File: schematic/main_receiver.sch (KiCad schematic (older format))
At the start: 52 parts, among them J7 CONN_01X05, J8 raspberry_pi_3_header, Q2 NXP 2N7002, Q3 NXP 2N7002, Q4 NXP 2N7002, Q5 NXP 2N7002, U7 SX1301, Y1 ASEMB-133.3MHZ

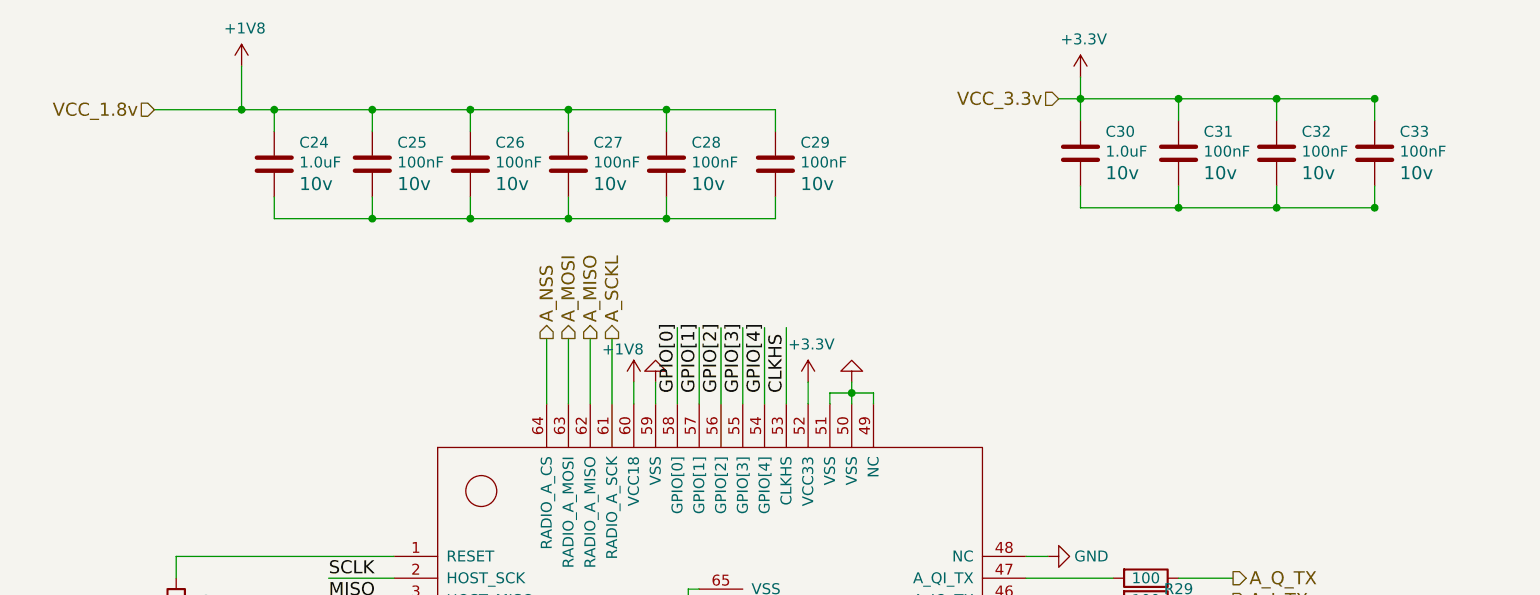
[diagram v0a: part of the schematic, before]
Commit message: Updates to schematic, components
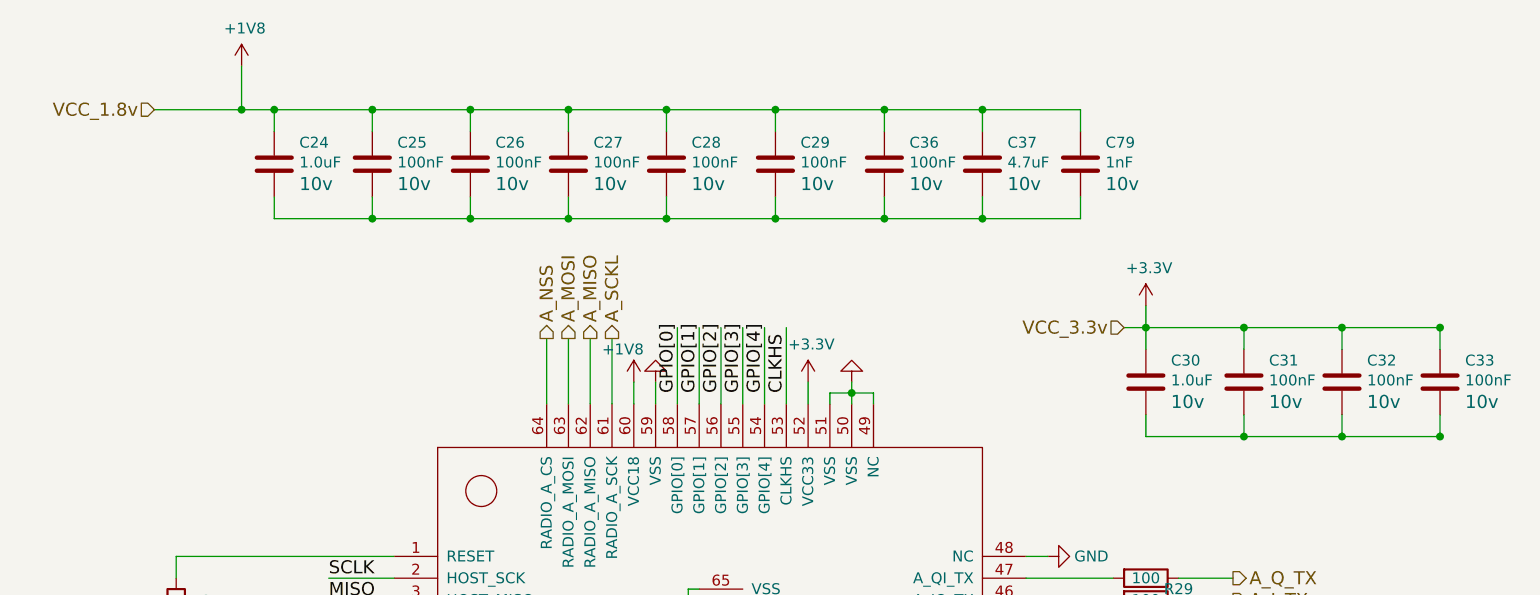
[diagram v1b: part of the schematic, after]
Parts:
- added C36: 100nF, symbol C
- added C37: 4.7uF, symbol C
- added C79: 1nF, symbol C
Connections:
- wire segments 191 -> 197
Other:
- moved on the sheet: C30, C31, C32, C33
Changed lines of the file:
@@
 L +3.3V #PWR055
 U 1 1 59B58145
-P 9000 900
-F 0 "#PWR055" H 9000 750 50  0001 C CNN
-F 1 "+3.3V" H 9015 1073 50  0000 C CNN
-F 2 "" H 9000 900 50  0001 C CNN
-F 3 "" H 9000 900 50  0001 C CNN
-	1    9000 900
-	1    0    0    -1
-$EndComp
-Text HLabel 8900 1000 0    60   Input ~ 0
+P 9300 1950
+F 0 "#PWR055" H 9300 1800 50  0001 C CNN
+F 1 "+3.3V" H 9315 2123 50  0000 C CNN
+F 2 "" H 9300 1950 50  0001 C CNN
+F 3 "" H 9300 1950 50  0001 C CNN
+	1    9300 1950
+	1    0    0    -1
+$EndComp
+Text HLabel 9200 2050 0    60   Input ~ 0
 VCC_3.3v
 Text HLabel 4750 1050 0    60   Input ~ 0
@@
 F 0 "C24" H 5415 1399 50  0000 L CNN
 F 1 "1.0uF" H 5415 1308 50  0000 L CNN
-F 2 "" H 5338 1150 50  0000 C CNN
+F 2 "" H 5338 1150 50  0001 C CNN
 F 3 "" H 5300 1300 50  0001 C CNN
 F 4 "10v" H 5415 1209 60  0000 L CNN "Voltage"
@@
 F 0 "C25" H 5865 1399 50  0000 L CNN
 F 1 "100nF" H 5865 1308 50  0000 L CNN
-F 2 "" H 5788 1150 50  0000 C CNN
+F 2 "" H 5788 1150 50  0001 C CNN
 F 3 "" H 5750 1300 50  0001 C CNN
 F 4 "10v" H 5865 1209 60  0000 L CNN "Voltage"
@@
 F 0 "C26" H 6315 1399 50  0000 L CNN
 F 1 "100nF" H 6315 1308 50  0000 L CNN
-F 2 "" H 6238 1150 50  0000 C CNN
+F 2 "" H 6238 1150 50  0001 C CNN
 F 3 "" H 6200 1300 50  0001 C CNN
 F 4 "10v" H 6315 1209 60  0000 L CNN "Voltage"
@@
 F 0 "C27" H 6765 1399 50  0000 L CNN
 F 1 "100nF" H 6765 1308 50  0000 L CNN
-F 2 "" H 6688 1150 50  0000 C CNN
+F 2 "" H 6688 1150 50  0001 C CNN
 F 3 "" H 6650 1300 50  0001 C CNN
 F 4 "10v" H 6765 1209 60  0000 L CNN "Voltage"
@@
 F 0 "C28" H 7215 1399 50  0000 L CNN
 F 1 "100nF" H 7215 1308 50  0000 L CNN
-F 2 "" H 7138 1150 50  0000 C CNN
+F 2 "" H 7138 1150 50  0001 C CNN
 F 3 "" H 7100 1300 50  0001 C CNN
 F 4 "10v" H 7215 1209 60  0000 L CNN "Voltage"
@@
 F 0 "C29" H 7715 1399 50  0000 L CNN
 F 1 "100nF" H 7715 1308 50  0000 L CNN
-F 2 "" H 7638 1150 50  0000 C CNN
+F 2 "" H 7638 1150 50  0001 C CNN
 F 3 "" H 7600 1300 50  0001 C CNN
 F 4 "10v" H 7715 1209 60  0000 L CNN "Voltage"
@@
 L C C30
 U 1 1 59B5D0C0
-P 9000 1250
-F 0 "C30" H 9115 1349 50  0000 L CNN
-F 1 "1.0uF" H 9115 1258 50  0000 L CNN
-F 2 "" H 9038 1100 50  0000 C CNN
-F 3 "" H 9000 1250 50  0001 C CNN
-F 4 "10v" H 9115 1159 60  0000 L CNN "Voltage"
-	1    9000 1250
+P 9300 2300
+F 0 "C30" H 9415 2399 50  0000 L CNN
+F 1 "1.0uF" H 9415 2308 50  0000 L CNN
+F 2 "" H 9338 2150 50  0001 C CNN
+F 3 "" H 9300 2300 50  0001 C CNN
+F 4 "10v" H 9415 2209 60  0000 L CNN "Voltage"
+	1    9300 2300
 	1    0    0    -1
 $EndComp
@@
 L C C31
 U 1 1 59B5D0C7
-P 9450 1250
-F 0 "C31" H 9565 1349 50  0000 L CNN
-F 1 "100nF" H 9565 1258 50  0000 L CNN
-F 2 "" H 9488 1100 50  0000 C CNN
-F 3 "" H 9450 1250 50  0001 C CNN
-F 4 "10v" H 9565 1159 60  0000 L CNN "Voltage"
-	1    9450 1250
+P 9750 2300
+F 0 "C31" H 9865 2399 50  0000 L CNN
+F 1 "100nF" H 9865 2308 50  0000 L CNN
+F 2 "" H 9788 2150 50  0001 C CNN
+F 3 "" H 9750 2300 50  0001 C CNN
+F 4 "10v" H 9865 2209 60  0000 L CNN "Voltage"
+	1    9750 2300
 	1    0    0    -1
 $EndComp
@@
 L C C32
 U 1 1 59B5D0CE
-P 9900 1250
-F 0 "C32" H 10015 1349 50  0000 L CNN
-F 1 "100nF" H 10015 1258 50  0000 L CNN
-F 2 "" H 9938 1100 50  0000 C CNN
-F 3 "" H 9900 1250 50  0001 C CNN
-F 4 "10v" H 10015 1159 60  0000 L CNN "Voltage"
-	1    9900 1250
+P 10200 2300
+F 0 "C32" H 10315 2399 50  0000 L CNN
+F 1 "100nF" H 10315 2308 50  0000 L CNN
+F 2 "" H 10238 2150 50  0001 C CNN
+F 3 "" H 10200 2300 50  0001 C CNN
+F 4 "10v" H 10315 2209 60  0000 L CNN "Voltage"
+	1    10200 2300
 	1    0    0    -1
 $EndComp
@@
 L C C33
 U 1 1 59B5D0D5
-P 10350 1250
-F 0 "C33" H 10465 1349 50  0000 L CNN
-F 1 "100nF" H 10465 1258 50  0000 L CNN
-F 2 "" H 10388 1100 50  0000 C CNN
-F 3 "" H 10350 1250 50  0001 C CNN
-F 4 "10v" H 10465 1159 60  0000 L CNN "Voltage"
-	1    10350 1250
+P 10650 2300
+F 0 "C33" H 10765 2399 50  0000 L CNN
+F 1 "100nF" H 10765 2308 50  0000 L CNN
+F 2 "" H 10688 2150 50  0001 C CNN
+F 3 "" H 10650 2300 50  0001 C CNN
+F 4 "10v" H 10765 2209 60  0000 L CNN "Voltage"
+	1    10650 2300
 	1    0    0    -1
 $EndComp
@@
 Connection ~ 3050 1150
 Wire Wire Line
-	4750 1050 7600 1050
+	4750 1050 9000 1050
 Wire Wire Line
 	5150 1050 5150 850
 Wire Wire Line
-	8900 1000 10350 1000
+	9200 2050 10650 2050
 Wire Wire Line
 	9300 4650 9200 4650
@@
 	7600 1550 7600 1450
 Wire Wire Line
-	5300 1550 7600 1550
+	5300 1550 9000 1550
 Wire Wire Line
 	5300 1550 5300 1450
@@
 Connection ~ 7100 1550
 Wire Wire Line
-	9450 1000 9450 1100
-Connection ~ 9450 1000
-Wire Wire Line
-	10350 1000 10350 1100
-Connection ~ 10350 1000
-Wire Wire Line
-	9900 1100 9900 1000
-Connection ~ 9900 1000
-Wire Wire Line
-	9000 1500 10350 1500
-Wire Wire Line
-	9450 1400 9450 1500
-Connection ~ 9450 1500
-Wire Wire Line
-	9900 1400 9900 1500
-Connection ~ 9900 1500
-Wire Wire Line
-	10350 1500 10350 1400
-Connection ~ 10350 1500
-Wire Wire Line
-	9000 900  9000 1100
-Connection ~ 9000 1000
-Wire Wire Line
-	9000 1500 9000 1400
+	9750 2050 9750 2150
+Connection ~ 9750 2050
+Wire Wire Line
+	10650 2050 10650 2150
+Connection ~ 10650 2050
+Wire Wire Line
+	10200 2150 10200 2050
+Connection ~ 10200 2050
+Wire Wire Line
+	9300 2550 10650 2550
+Wire Wire Line
+	9750 2450 9750 2550
+Connection ~ 9750 2550
+Wire Wire Line
+	10200 2450 10200 2550
+Connection ~ 10200 2550
+Wire Wire Line
+	10650 2550 10650 2450
+Connection ~ 10650 2550
+Wire Wire Line
+	9300 1950 9300 2150
+Connection ~ 9300 2050
+Wire Wire Line
+	9300 2550 9300 2450
 Wire Wire Line
 	7050 2300 7050 2400
@@
 $EndComp
 NoConn ~ 1450 2950
+$Comp
+L C C36
+U 1 1 59B464FB
+P 8100 1300
+F 0 "C36" H 8215 1399 50  0000 L CNN
+F 1 "100nF" H 8215 1308 50  0000 L CNN
+F 2 "" H 8138 1150 50  0001 C CNN
+F 3 "" H 8100 1300 50  0001 C CNN
+F 4 "10v" H 8215 1209 60  0000 L CNN "Voltage"
+	1    8100 1300
+	1    0    0    -1
+$EndComp
+Wire Wire Line
+	8100 1050 8100 1150
+Connection ~ 7600 1050
+Wire Wire Line
+	8100 1550 8100 1450
+Connection ~ 7600 1550
+$Comp
+L C C37
+U 1 1 59B475A8
+P 8550 1300
+F 0 "C37" H 8665 1399 50  0000 L CNN
+F 1 "4.7uF" H 8665 1308 50  0000 L CNN
+F 2 "" H 8588 1150 50  0001 C CNN
+F 3 "" H 8550 1300 50  0001 C CNN
+F 4 "10v" H 8665 1209 60  0000 L CNN "Voltage"
+	1    8550 1300
+	1    0    0    -1
+$EndComp
+$Comp
+L C C79
+U 1 1 59B47640
+P 9000 1300
+F 0 "C79" H 9115 1399 50  0000 L CNN
+F 1 "1nF" H 9115 1308 50  0000 L CNN
+F 2 "" H 9038 1150 50  0001 C CNN
+F 3 "" H 9000 1300 50  0001 C CNN
+F 4 "10v" H 9115 1209 60  0000 L CNN "Voltage"
+	1    9000 1300
+	1    0    0    -1
+$EndComp
+Wire Wire Line
+	8550 1550 8550 1450
+Connection ~ 8100 1550
+Wire Wire Line
+	9000 1550 9000 1450
+Connection ~ 8550 1550
+Wire Wire Line
+	9000 1050 9000 1150
+Connection ~ 8100 1050
+Wire Wire Line
+	8550 1050 8550 1150
+Connection ~ 8550 1050
 $EndSCHEMATC
